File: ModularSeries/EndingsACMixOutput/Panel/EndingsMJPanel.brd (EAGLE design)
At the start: 48.5 x 100 mm, 12 parts

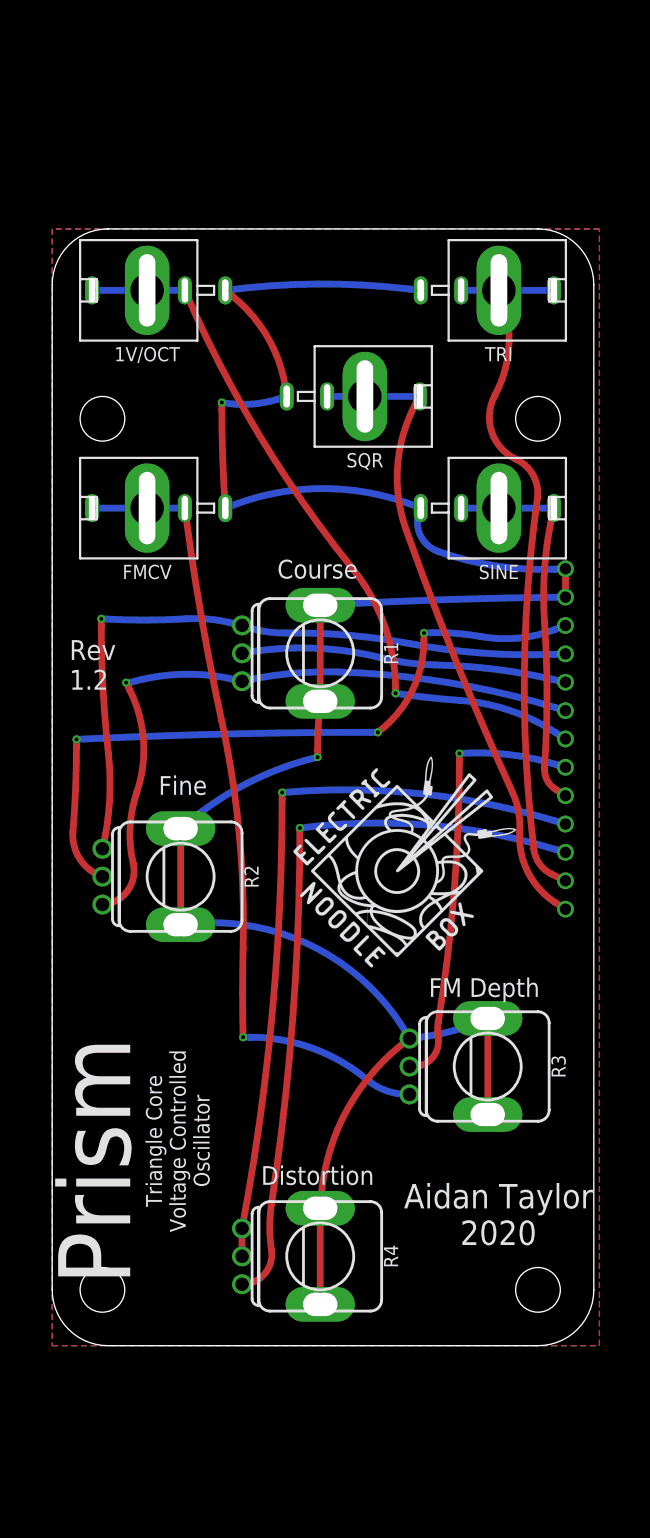
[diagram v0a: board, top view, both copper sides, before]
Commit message: Fields added and various updates to designs
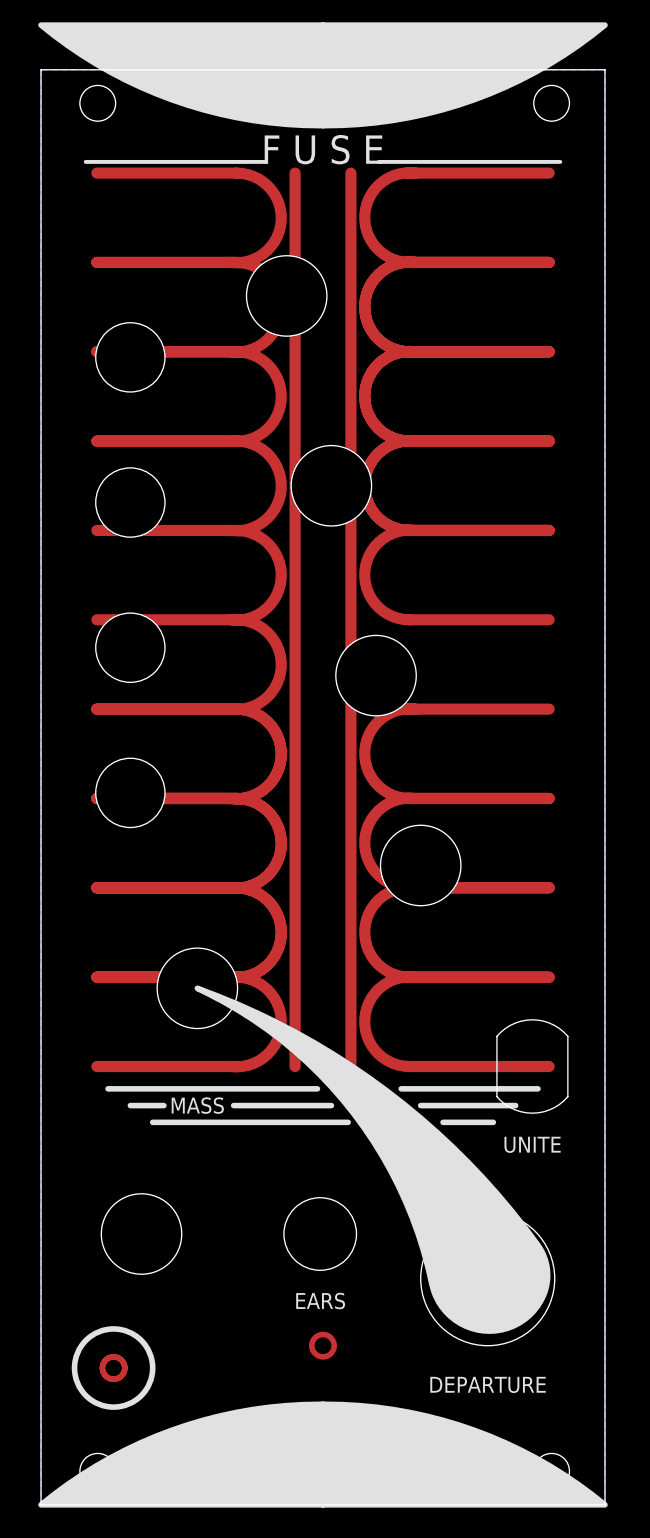
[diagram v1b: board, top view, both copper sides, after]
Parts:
- removed 1V/OCT, FMCV, SINE, SQR, TRI: COMBI-JACKCINCHNANA, ElectricNoodleBox:NEWCOMBOJACK_PANEL
- removed BOARD1: PRISM_LINK, ElectricNoodleBox:PRISM
- removed R1, R2, R3, R4: B100K, ElectricNoodleBox:ALPHA_RV09_9MMPOT
- removed U$1, U$2: (no value), ElectricNoodleBox:LOGO20X20
- added E$10, E$11, E$2, E$7, E$8, E$9: (no value), ElectricNoodleBox:ALPHA9MM_POT_CUTOUT
- added E$12: (no value), ElectricNoodleBox:MINIJACK_M6_CUTOUT
- added E$13: (no value), ElectricNoodleBox:NEUTRIK_6.35_CUTOUT
- added E$14: (no value), ElectricNoodleBox:LOGO20X20
- added E$6: (no value), ElectricNoodleBox:CINCH_BANANA_CUTOUT
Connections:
- removed net AGND: 1V/OCT.S, BOARD1.GNDA, BOARD1.GNDB, FMCV.S, R1.LUGL, R1.LUGR, R2.LUGL, R2.LUGR, R3.C1, R3.LUGL, R3.LUGR, R4.LUGL, R4.LUGR, SINE.S, SQR.S, TRI.S
- removed net N$1: 1V/OCT.CONN, 1V/OCT.T1, 1V/OCT.T2, BOARD1.CVA
- removed net N$10: BOARD1.SIN, SINE.CONN, SINE.T1, SINE.T2
- removed net N$11: BOARD1.TRI, TRI.CONN, TRI.T1, TRI.T2
- removed net N$12: BOARD1.SQR, SQR.CONN, SQR.T1, SQR.T2
- removed net N$2: BOARD1.F1, R1.C1, R2.C1
- removed net N$3: BOARD1.F3, R1.C3, R2.C3
- removed net N$4: BOARD1.F2, R1.C2
- removed net N$5: BOARD1.FINE, R2.C2
- removed net N$6: FMCV.CONN, FMCV.T1, FMCV.T2, R3.C3
- removed net N$7: BOARD1.CVB, R3.C2
- removed net N$8: BOARD1.DIST1, R4.C1, R4.C2
- removed net N$9: BOARD1.DIST2, R4.C3
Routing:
- net AGND: track 202.4 -> 0.00 mm, vias 2 -> 0
- net S$2: track 0.00 -> 80.0 mm
- net S$1: track 0.00 -> 80.0 mm
- net N$6: track 71.8 -> 0.00 mm, vias 1 -> 0
- net N$8: track 67.2 -> 0.00 mm, vias 1 -> 0
- net N$9: track 65.8 -> 0.00 mm, vias 1 -> 0
- net N$1: track 65.1 -> 0.00 mm, vias 1 -> 0
- net N$11: track 63.3 -> 0.00 mm
- net N$5: track 62.7 -> 0.00 mm, vias 3 -> 0
- net N$2: track 62.4 -> 0.00 mm, vias 1 -> 0
- net N$3: track 60.6 -> 0.00 mm, vias 1 -> 0
- net N$12: track 57.4 -> 0.00 mm
- net N$7: track 38.7 -> 0.00 mm, vias 1 -> 0
- net N$10: track 34.8 -> 0.00 mm
- net N$4: track 29.1 -> 0.00 mm
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- added copper zone on layer 16, net GND
- removed copper zone on layer 1, net AGND
- removed copper zone on layer 16, net AGND
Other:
- board size 48.5 x 100 mm -> 50.5 x 128.5 mm
- board text added: "DEPARTURE"
- board text added: "E N D I N G S"
- board text added: "EARS"
- board text added: "F U S E"
- board text added: "MASS"
- board text added: "UNITE"
- board text removed: "Aidan Taylor 2020"
- board text removed: "Course"
- board text removed: "Distortion"
- board text removed: "FM Depth"
- board text removed: "Fine"
- board text removed: "Prism"
- board text removed: "Rev 1.2"
- board text removed: "Triangle Core Voltage Controlled Oscillator"
